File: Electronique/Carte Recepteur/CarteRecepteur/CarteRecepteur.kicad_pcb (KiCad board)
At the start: 2 copper layers, 27 x 62 mm, 3 parts, among them J1 Conn_02x04_Odd_Even_MountingP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

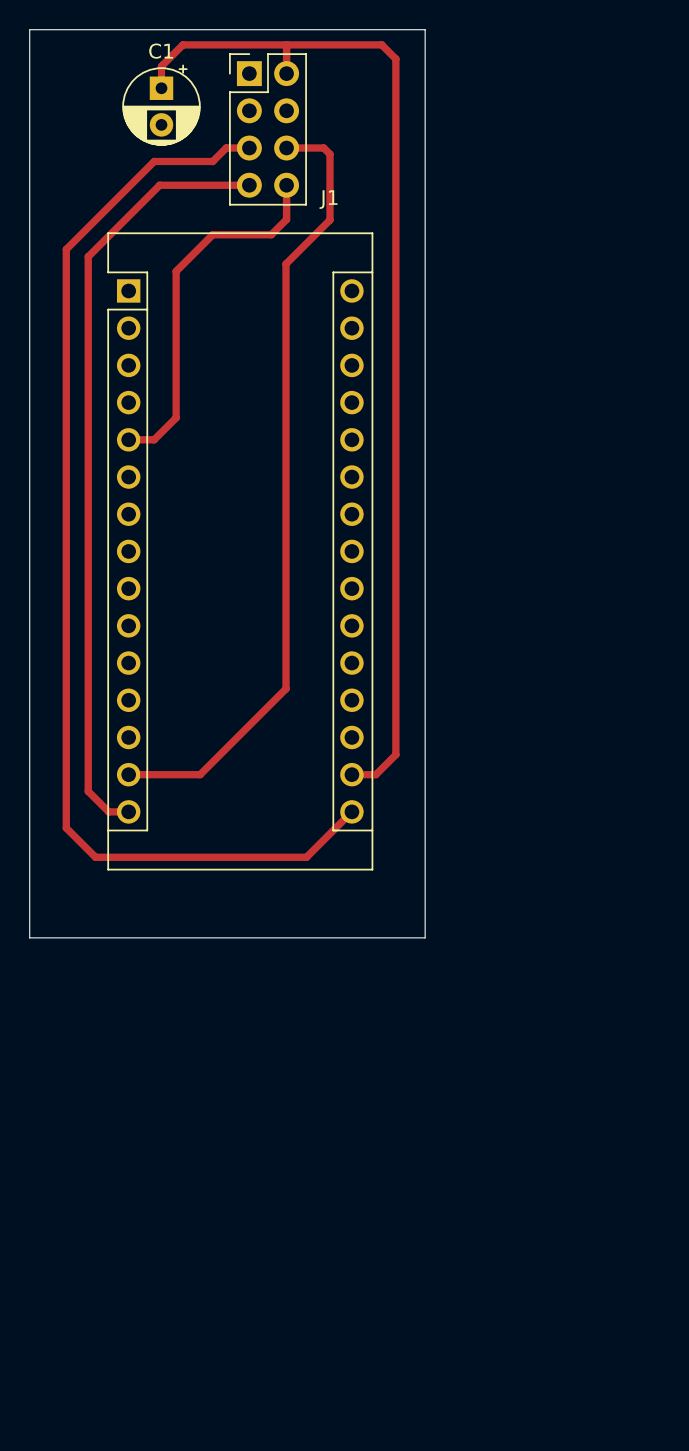
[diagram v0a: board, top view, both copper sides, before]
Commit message: pcb recepteur
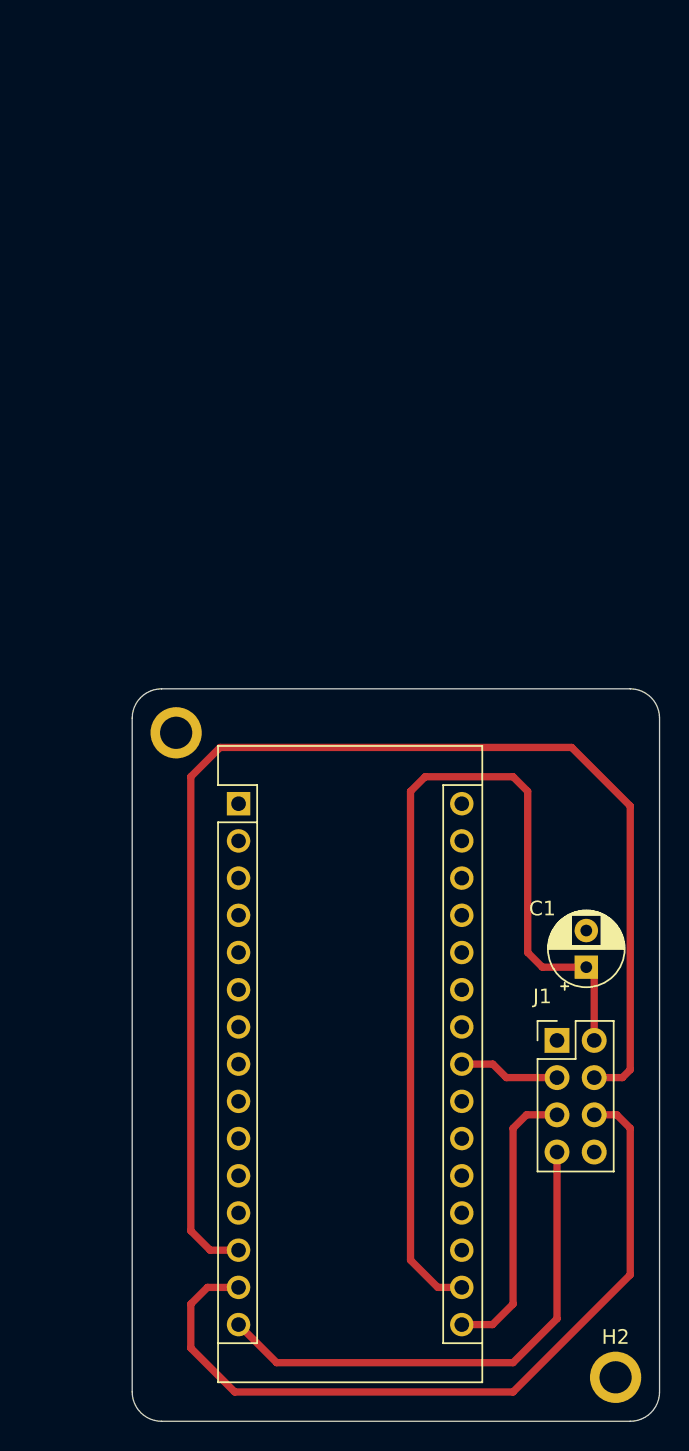
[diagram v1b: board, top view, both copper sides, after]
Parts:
- added H1: MountingHole, MountingHole:MountingHole_2.2mm_M2_ISO7380_Pad, F.Cu at (108.0, 48.0)
- added H2: MountingHole, MountingHole:MountingHole_2.2mm_M2_ISO7380_Pad, F.Cu at (138.0, 92.0)
- moved J1 69.3 mm to (134.0, 69.0)
- moved C1 66.6 mm to (136.0, 64.0), turned to 90 degrees
- moved A1 35.8 mm to (112.3, 52.8)
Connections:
- A1 pad 12: /CE -> (no net)
- A1 pad 23: (no net) -> /CE
- A1 pad 5: /IRQ -> (no net)
- J1 pad 8: /IRQ -> (no net)
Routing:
- net /CS: track 0.00 -> 88.0 mm
- net /SCK: track 76.5 -> 19.5 mm
- net /IRQ: track 25.2 -> 0.00 mm
- net /MISO: track 52.9 -> 35.4 mm
- net /CE: track 0.00 -> 6.88 mm
- net +3V3: track 71.5 -> 65.7 mm
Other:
- board size 27 x 62 mm -> 36 x 50 mm
